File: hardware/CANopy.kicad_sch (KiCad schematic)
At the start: 11 parts, among them J1 RPi_GPIO, J2 CAN0, J3 CAN1, J4 CAN2, U7 AT24C32

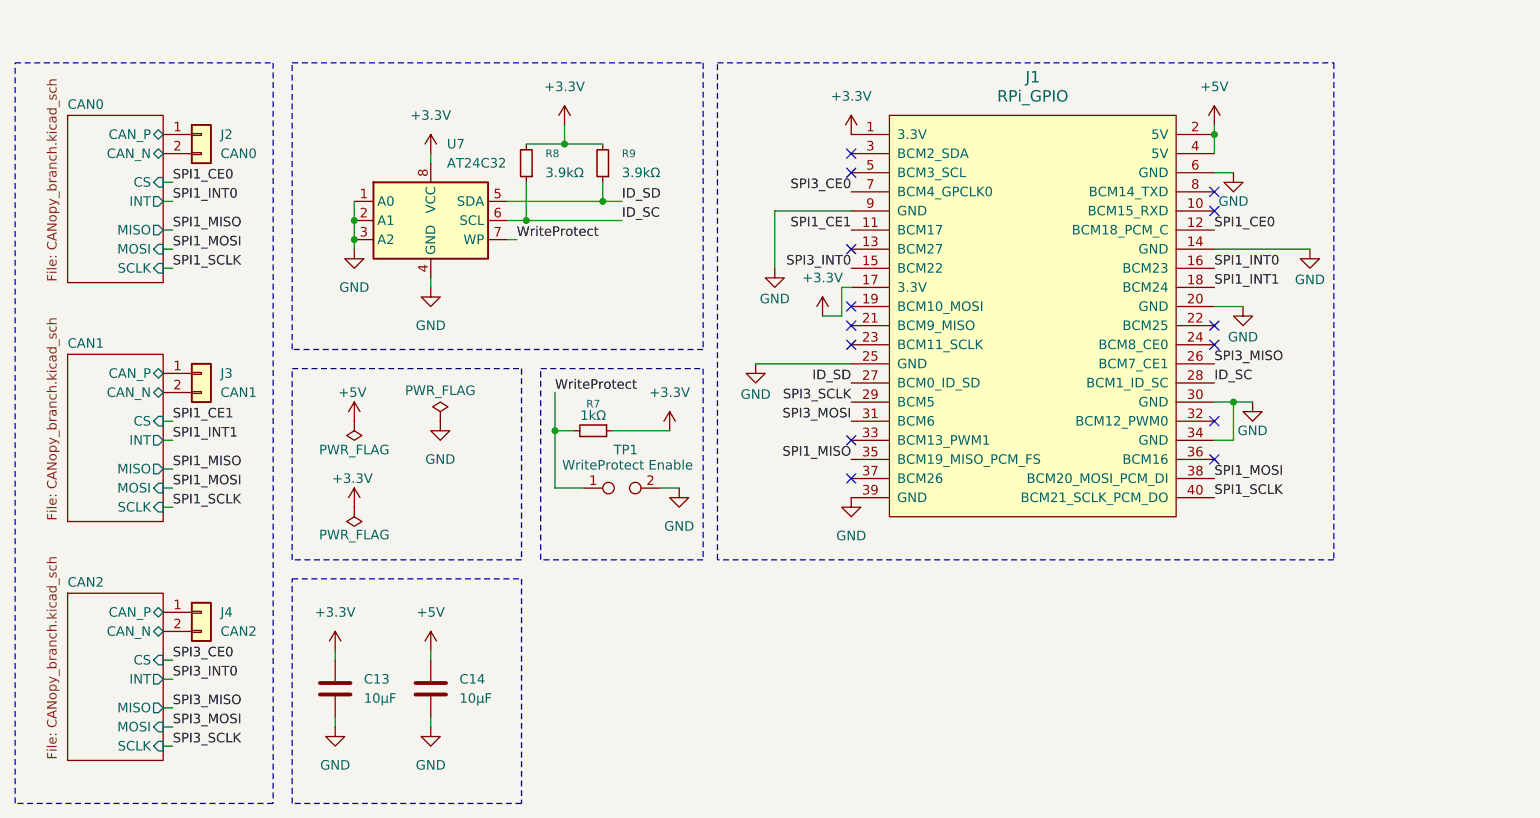
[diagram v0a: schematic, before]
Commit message: feat: first pass reroute
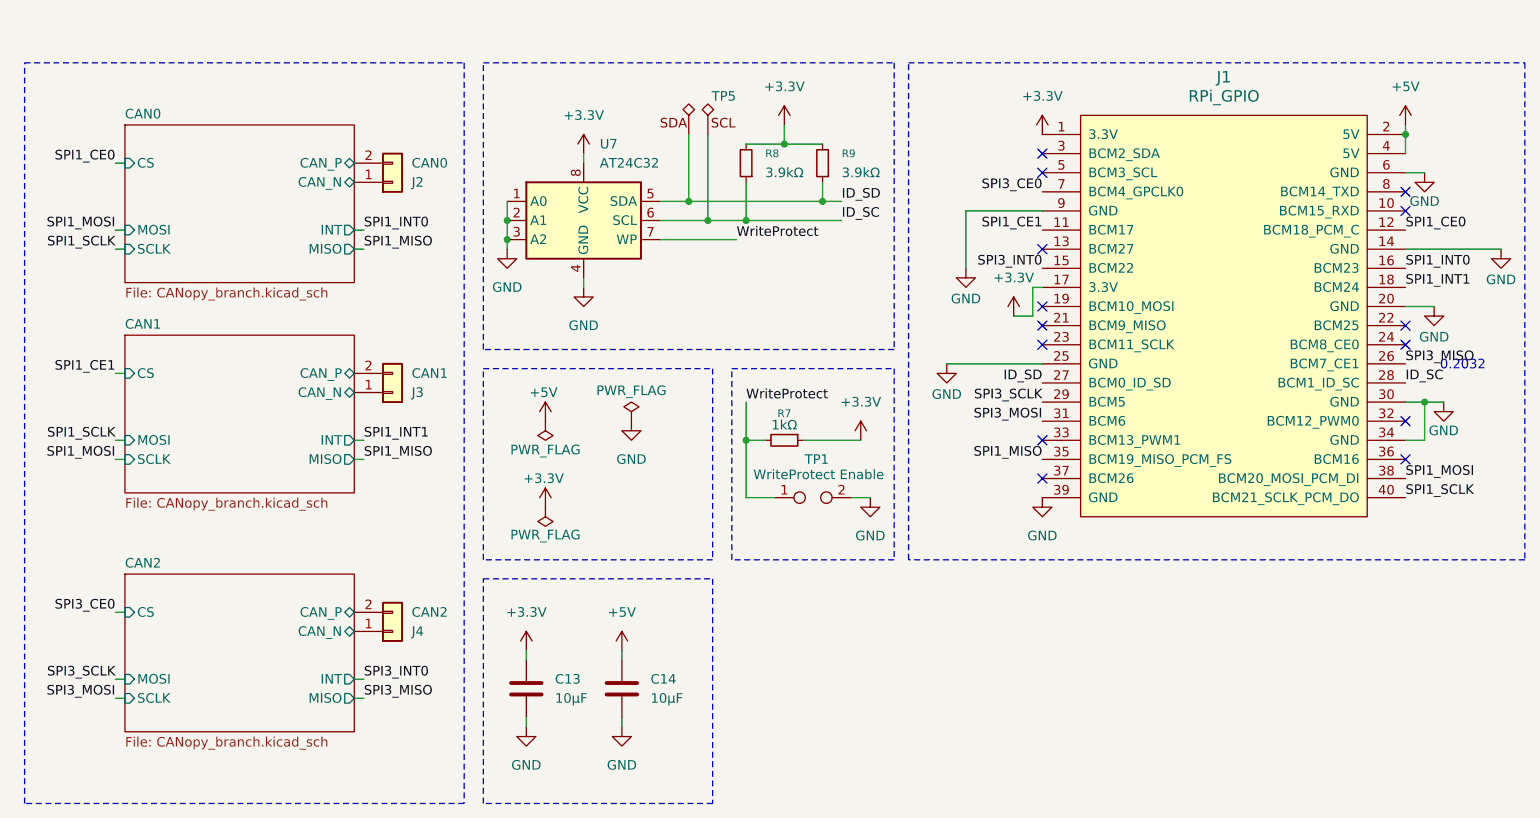
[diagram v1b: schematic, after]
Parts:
- added TP5: SDA SCL, symbol Connector:TestPoint_Alt
- J2, J3, J4: footprint Degson:SHDRRA2W80P0X350_1X2_780X920X722P -> Degson:CONN-TH_DG500-5.08-02P-14-00A-H
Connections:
- net CAN0/CAN_N: now also J2.1 (Pin_1); no longer J2.2 (Pin_2)
- net CAN0/CAN_P: now also J2.2 (Pin_2); no longer J2.1 (Pin_1)
- net CAN1/CAN_N: now also J3.1 (Pin_1); no longer J3.2 (Pin_2)
- net CAN1/CAN_P: now also J3.2 (Pin_2); no longer J3.1 (Pin_1)
- net CAN2/CAN_N: now also J4.1 (Pin_1); no longer J4.2 (Pin_2)
- net CAN2/CAN_P: now also J4.2 (Pin_2); no longer J4.1 (Pin_1)
- net ID_SC: now also TP5.1 (TX)
- net ID_SD: now also TP5.1 (TX)
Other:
- note added: "0.2032"
- moved on the sheet: C13, C14, J1, J2, J3, J4, R7, R8, R9, TP1, U7
